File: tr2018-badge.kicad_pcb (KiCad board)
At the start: 2 copper layers, 70.4 x 53.3 mm, 20 parts, among them J1 Conn_01x02, J2 Conn_01x02, SW1 SW_SPDT, SW3 SW_Push, SW4 SW_Push, SW5 SW_SPDT, U1 ESP-12F, X1 Badgelife_shitty_connector

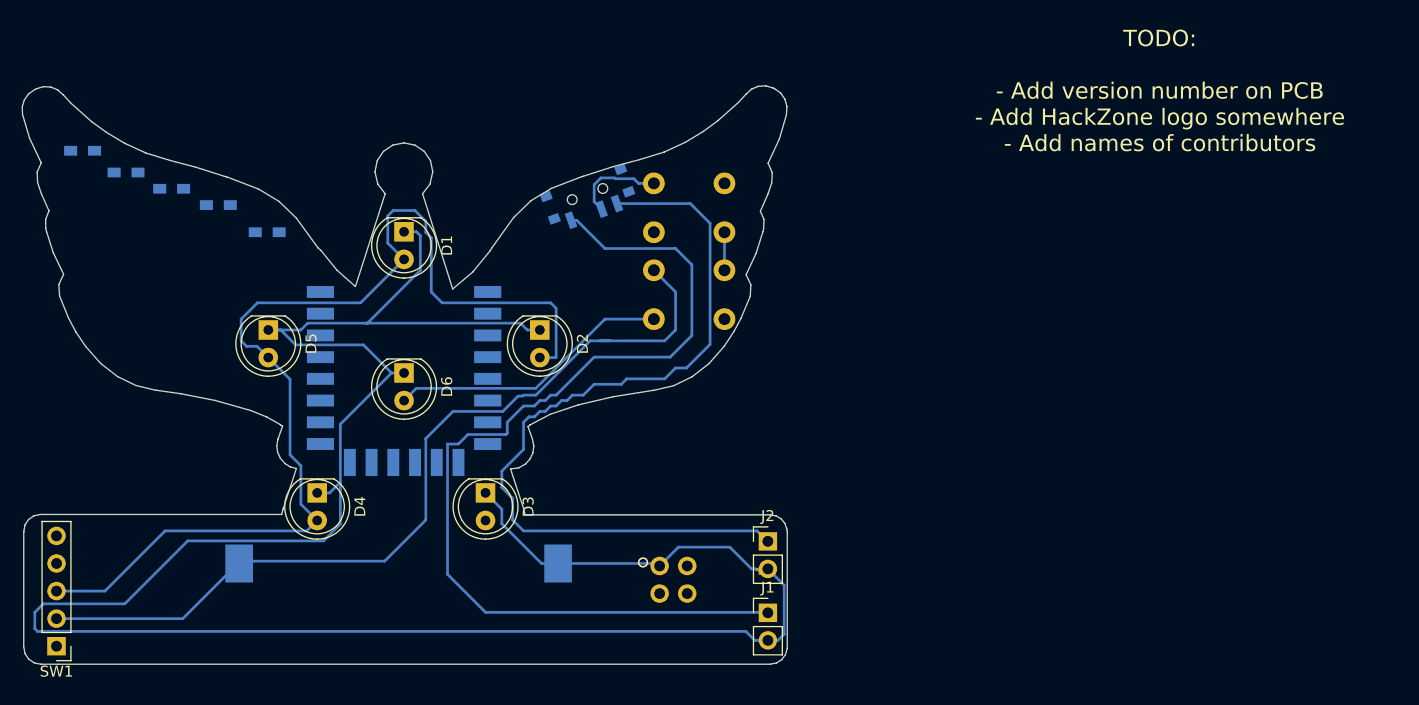
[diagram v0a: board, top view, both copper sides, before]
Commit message: Bump to rev 1.0.0
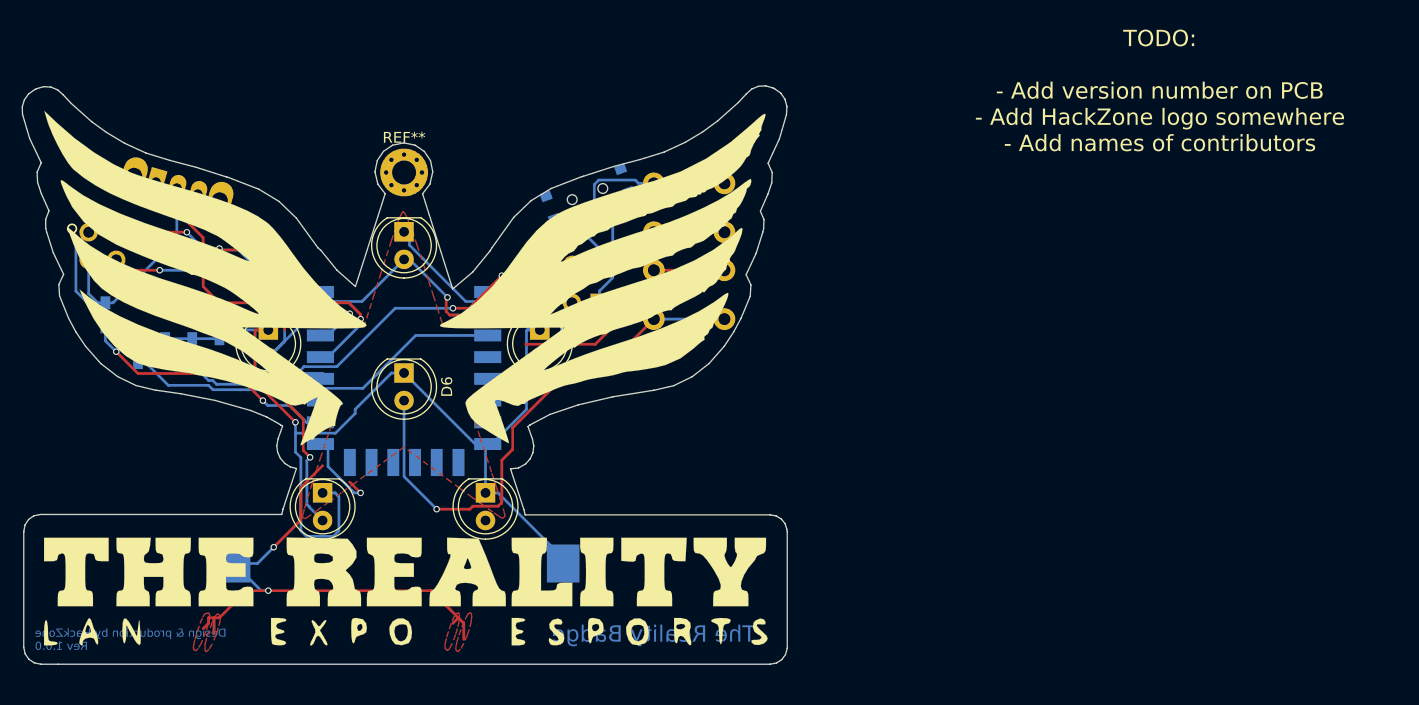
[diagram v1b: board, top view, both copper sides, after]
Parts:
- added G***: LOGO, modules:fill_mask, F.Cu at (147.0, 94.0)
- added REF**: MountingHole_2.2mm_M2_Pad_Via, Mounting_Holes:MountingHole_2.2mm_M2_Pad_Via, F.Cu at (147.0, 75.5)
- added Wings: LOGO, modules:wingstext, F.Cu at (147.0, 94.0)
- BT1: footprint Battery_Holders:Keystone_1058_1x2032-CoinCell -> BatteryHolder:Keystone_1058_1x2032-CoinCell
- J1, J2: moved to B.Cu
- R5: value 10k -> 10k (all opt.)
- SW1: footprint Pin_Headers:Pin_Header_Straight_1x05_Pitch2.54mm -> modules:SW_CuK_OS102011MA1QN1_SPDT_Angled; moved to B.Cu
- SW5 (opt.): renamed from SW5
- U1: value ESP-12F -> ESP-12F (opt.)
- X1: value Badgelife_shitty_connector -> Defcon Shitty AddOn (opt.) >
- moved X1 60.9 mm to (119.2, 82.3)
- moved SW1 43.7 mm to (124.2, 76.4), turned to 344 degrees
- moved J1 35.6 mm to (165.0, 84.0), turned to 90 degrees
- moved J2 26.9 mm to (165.0, 87.5), turned to 90 degrees
- moved R4 16.4 mm to (122.5, 91.9), turned to 270 degrees
- moved R5 15.2 mm to (119.5, 88.6), turned to 270 degrees
- moved R3 14.9 mm to (125.0, 91.9), turned to 270 degrees
- moved R2 13.6 mm to (127.5, 91.9), turned to 90 degrees
- moved R1 11.8 mm to (130.0, 91.9), turned to 90 degrees
- moved D4 0.50 mm to (139.5, 105.0)
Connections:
- SW1 pad 1: (no net) -> Net-(SW1-Pad1)
- U1 pad 15: (no net) -> Net-(U1-Pad15)
- U1 pad 16: (no net) -> Net-(U1-Pad16)
- U1 pad 17: (no net) -> Net-(U1-Pad17)
- U1 pad 18: (no net) -> Net-(U1-Pad18)
- U1 pad 19: (no net) -> Net-(U1-Pad19)
- U1 pad 2: (no net) -> Net-(U1-Pad2)
- U1 pad 20: (no net) -> Net-(U1-Pad20)
- U1 pad 21: (no net) -> Net-(U1-Pad21)
- U1 pad 22: (no net) -> Net-(U1-Pad22)
- U1 pad 4: (no net) -> Net-(U1-Pad4)
- U1 pad 5: (no net) -> Net-(U1-Pad5)
- U1 pad 6: (no net) -> Net-(U1-Pad6)
- U1 pad 7: (no net) -> Net-(U1-Pad7)
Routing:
- net Net-(J1-Pad1): track 89.5 -> 5.20 mm
- net VCC: track 210.4 -> 132.3 mm, vias 0 -> 1
- net Net-(J2-Pad1): track 75.2 -> 9.80 mm
- net GND: track 83.2 -> 126.2 mm, vias 0 -> 3
- net Net-(R1-Pad1): track 0.00 -> 32.7 mm, vias 0 -> 2
- net SDA: track 0.00 -> 30.8 mm, vias 0 -> 3
- net Net-(R2-Pad1): track 0.00 -> 29.6 mm
- net SCL: track 0.00 -> 26.4 mm, vias 0 -> 3
- net Net-(R5-Pad2): track 0.00 -> 24.9 mm, vias 0 -> 2
- net Net-(D1-Pad2): track 99.6 -> 76.8 mm, vias 0 -> 3
- net Net-(D6-Pad2): track 26.1 -> 48.4 mm, vias 0 -> 1
- net Net-(R4-Pad2): track 0.00 -> 18.9 mm
- net FLASH_EN: track 0.00 -> 17.1 mm
- net Net-(SW4-Pad2): track 8.50 -> 14.8 mm
- net (no net): track 0.72 -> 0.00 mm
- added copper zone on F.Cu, net GND
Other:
- board text added: "< all opt. ^"
- board text added: "Design & production by HackZone Rev 1.0.0"
- board text added: "The Reality Badge"
